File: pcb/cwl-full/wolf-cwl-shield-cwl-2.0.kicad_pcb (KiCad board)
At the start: 2 copper layers, 170.8 x 75.7 mm, 30 parts, among them J1 UEXT, J2 OpenTherm, J3 OLED_0.96, J4 OLED_1.3, Q1 BC858A, SW1 EC12E24204A9, U1 PC817, U2 PC817

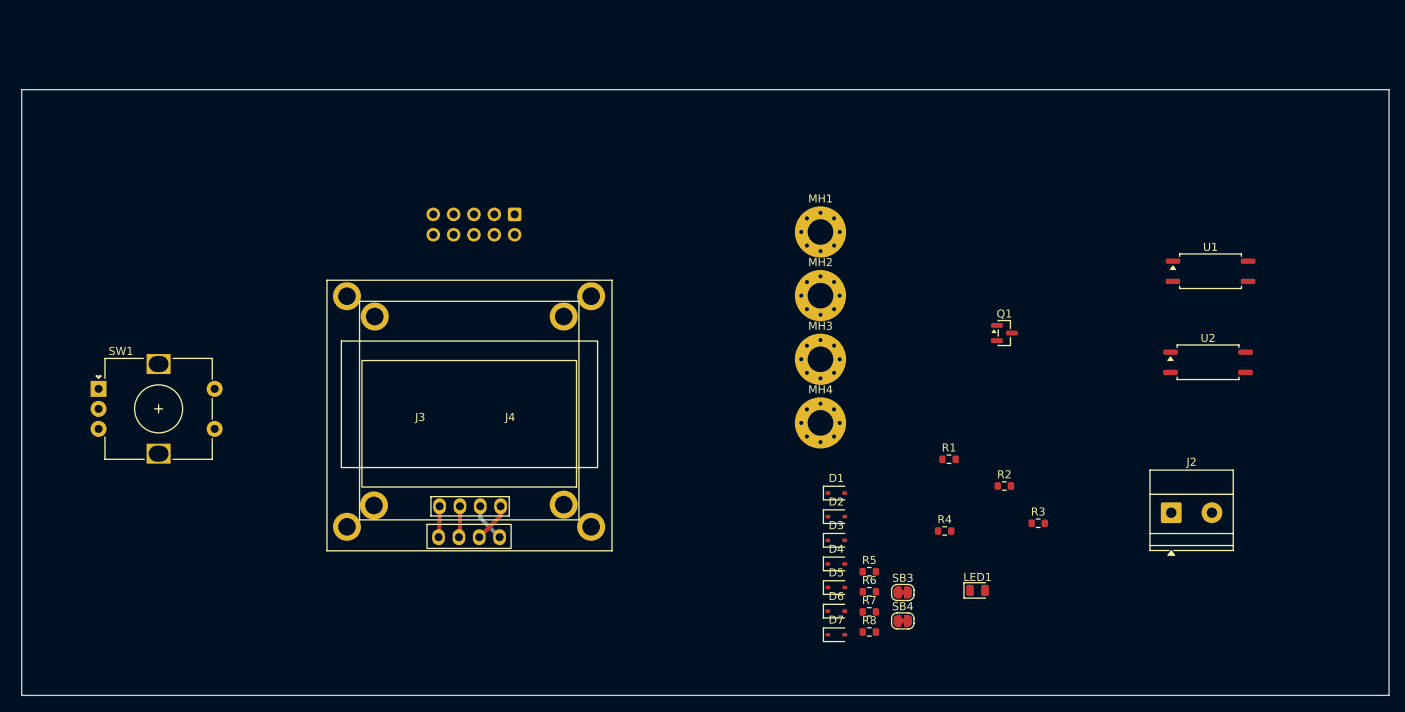
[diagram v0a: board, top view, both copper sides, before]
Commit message: new pcb
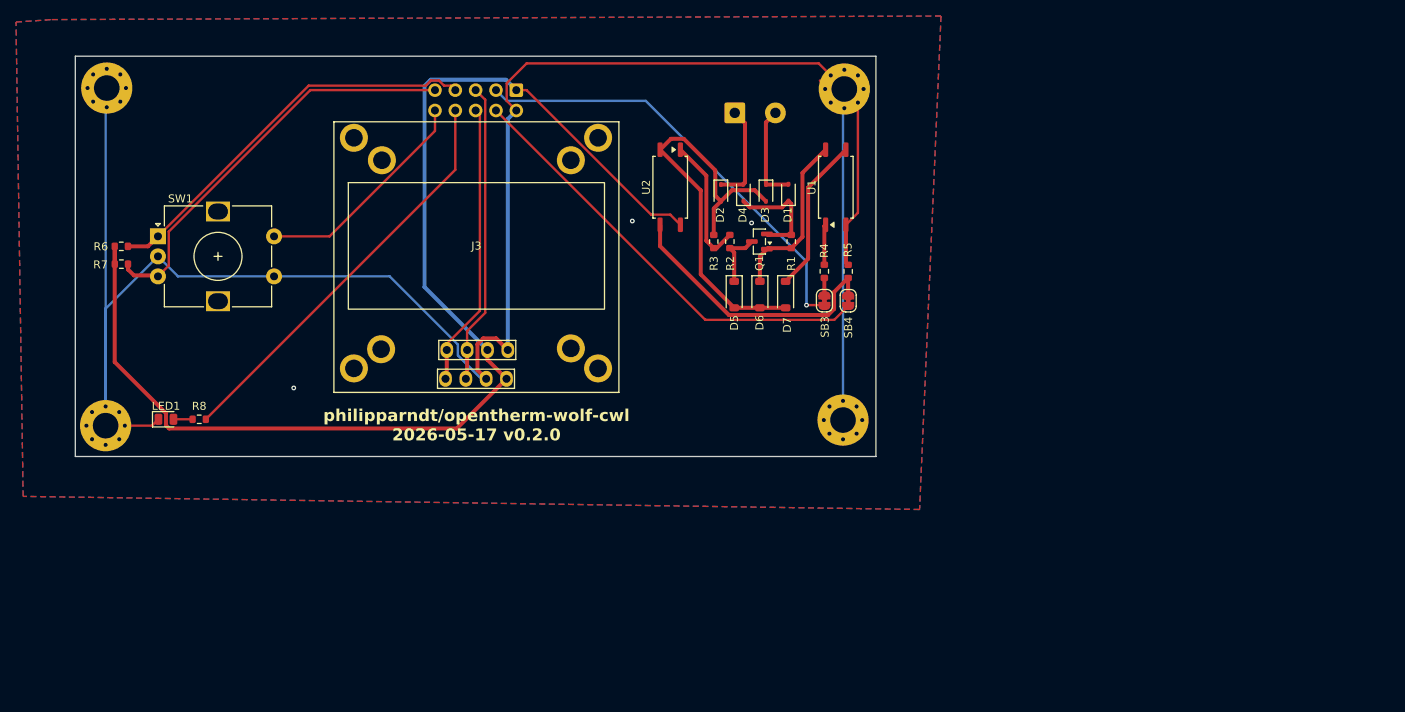
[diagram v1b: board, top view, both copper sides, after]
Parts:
- removed J4: OLED_1.3, SSD1306:128x64OLED-MountingHoles-Large
- D5, D6, D7: footprint Diode_SMD:D_SOD-323 -> Diode_SMD:D_SOD-123
- J2: moved to B.Cu
- J3: value OLED_0.96 -> OLED; footprint SSD1306:128x64OLED-MountingHoles -> SSD1306:128x64OLED-MountingHoles-Combined
- moved LED1 103.6 mm to (51.2, 105.6)
- moved R7 103.0 mm to (45.6, 86.2), turned to 180 degrees
- moved R6 102.9 mm to (45.6, 84.0)
- moved MH1 90.9 mm to (43.8, 64.2)
- moved MH3 89.7 mm to (43.6, 106.4)
- moved R8 87.8 mm to (55.3, 105.6), turned to 180 degrees
- moved J2 73.9 mm to (122.2, 67.3)
- moved U2 70.6 mm to (114.1, 76.6), turned to -90 degrees
- moved J3 58.4 mm to (72.1, 68.4), turned to 0 degrees
- moved R3 53.7 mm to (119.6, 83.4), turned to 90 degrees
- moved D4 48.5 mm to (120.5, 77.3), turned to -90 degrees
- moved U1 48.0 mm to (134.8, 76.6), turned to 90 degrees
- moved R2 45.9 mm to (121.6, 83.4), turned to -90 degrees
- moved D3 44.3 mm to (126.1, 77.3), turned to -90 degrees
- moved D7 43.0 mm to (128.6, 90.0), turned to -90 degrees
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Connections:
- J2 pad 1: OT+ -> OT-
- J2 pad 2: OT- -> OT+
- J3 pad 1: GND -> +3V3
- J3 pad 2: +3V3 -> GND
- R4 pad 2: OT_RX_SIG -> OT_TX_SIG
- R5 pad 1: OT_TX_SIG -> OT_RX_SIG
- R6 pad 1: ENC_CLK -> +3V3
- R6 pad 2: +3V3 -> ENC_CLK
- U2 pad 3: OT_TX_SIG -> OT_RX_SIG
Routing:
- net GND: track 4.97 -> 272.3 mm, vias 0 -> 3
- net +3V3: track 4.86 -> 153.1 mm
- net UEXT_RXD: track 0.00 -> 55.5 mm
- net UEXT_TXD: track 0.00 -> 55.4 mm, vias 0 -> 1
- net Net-(D3-A): track 0.00 -> 54.6 mm
- net ENC_DT: track 0.00 -> 51.5 mm
- net LED_GPIO: track 0.00 -> 51.5 mm
- net ENC_CLK: track 0.00 -> 50.0 mm
- net OT_RX_SIG: track 0.00 -> 35.1 mm
- net SCL: track 3.92 -> 37.6 mm
- net SDA: track 3.92 -> 35.5 mm
- net ENC_SW: track 0.00 -> 28.1 mm
- net Net-(D6-K): track 0.00 -> 21.6 mm
- net Net-(D7-K): track 0.00 -> 19.6 mm
- net Net-(R2-Pad1): track 0.00 -> 16.7 mm
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- added copper zone on B.Cu, net GND
- added copper zone on F.Cu, net GND
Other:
- board size 170.8 x 75.7 mm -> 100 x 50 mm
- board text added: "philipparndt/opentherm-wolf-cwl 2026-05-17 v0.2.0"
